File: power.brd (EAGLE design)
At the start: 136 x 136 mm, 35 parts, among them CN1 21700, CN2 21700, CN3 21700, CN4 21700, CN5 15PIN 0.5MM, Q6 IRLML6244, Q7 IRLML6244, U17 MAX17320G20+

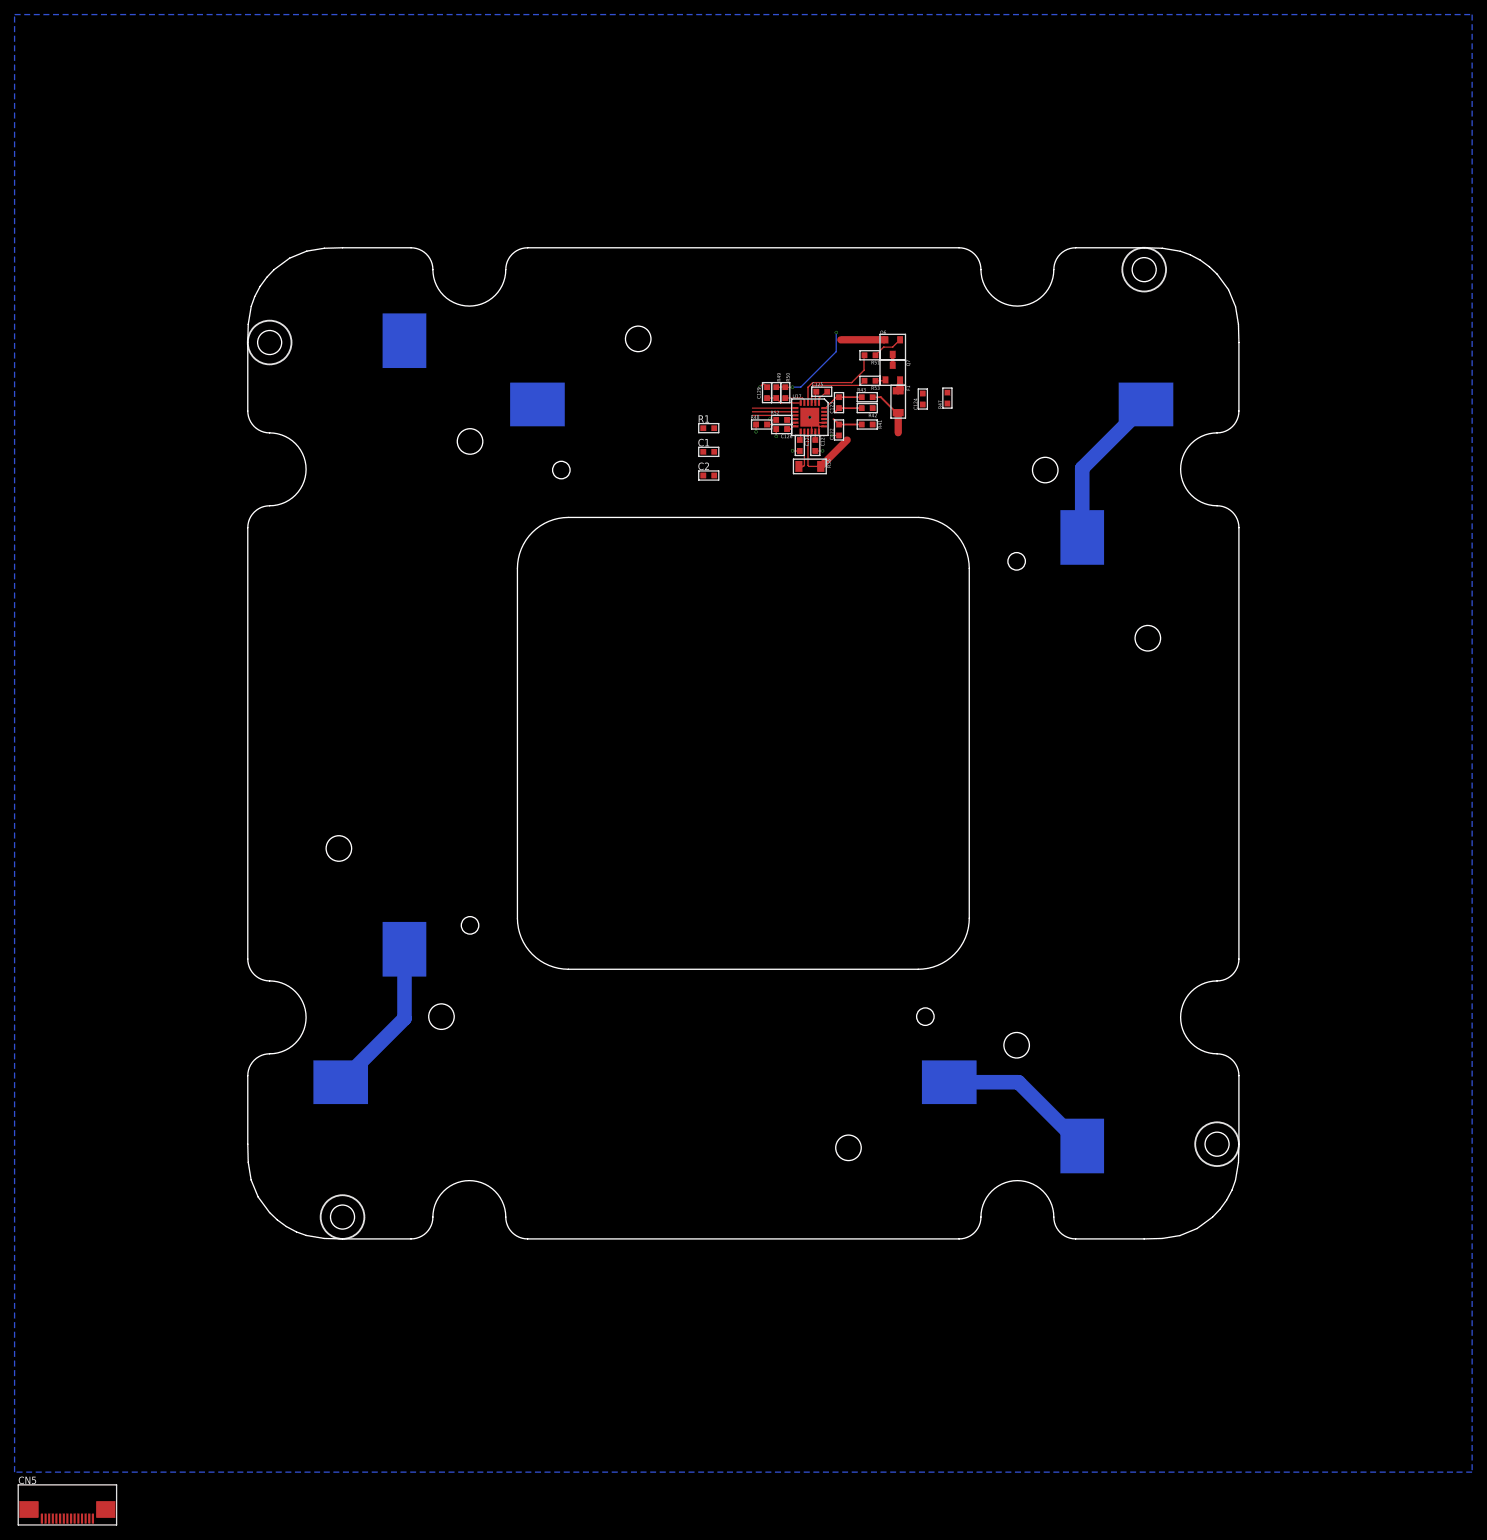
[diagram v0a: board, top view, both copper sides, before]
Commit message: Mech design and layout
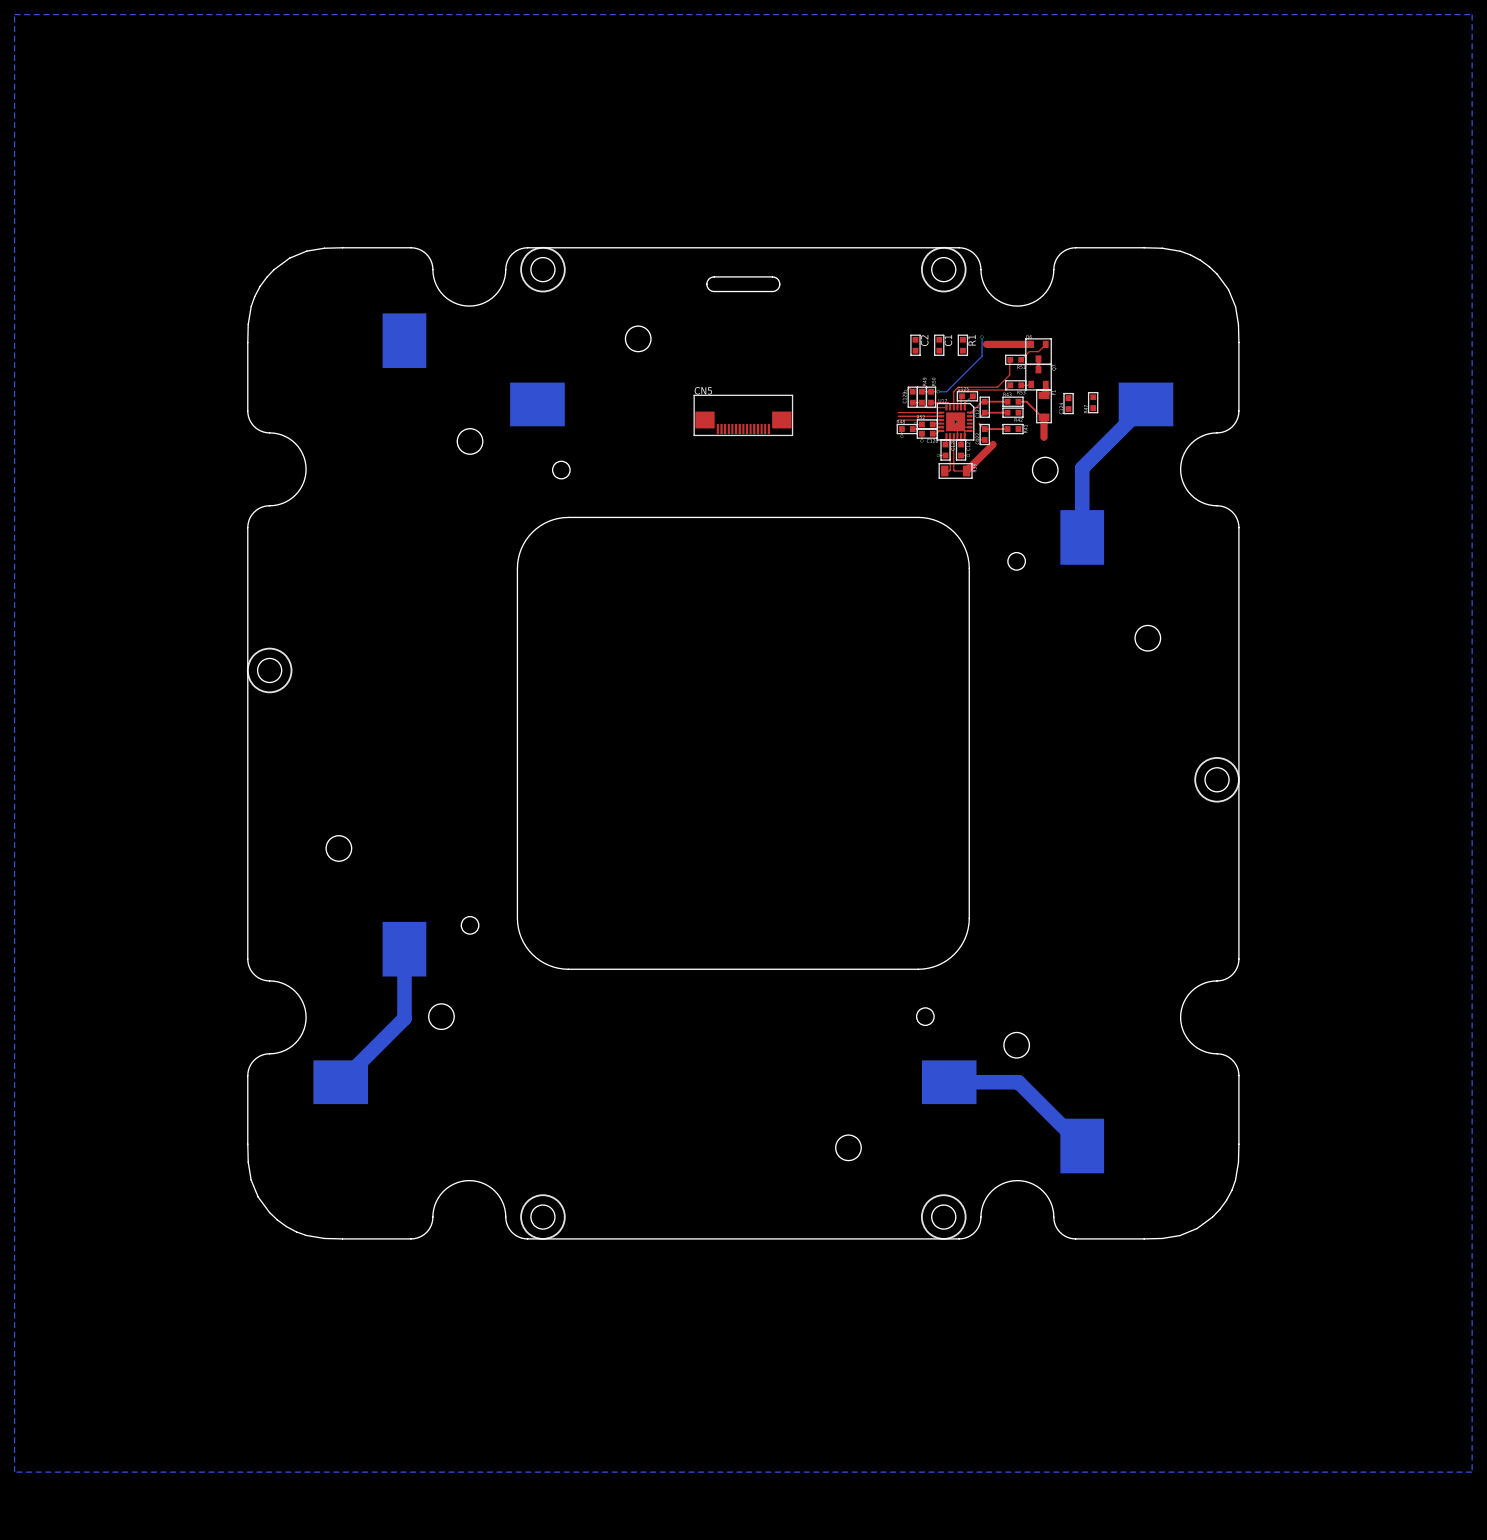
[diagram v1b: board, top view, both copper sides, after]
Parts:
- added MECH5, MECH6: 6mm x 3mm, MISC:MOUNTHOLE_6X3
- moved CN5 175.9 mm to (0.00, 45.0)
- moved MECH2 38.8 mm to (-27.5, 65.0)
- moved MECH4 38.8 mm to (27.5, -65.0)
- moved R1 36.7 mm to (30.1, 54.6), turned to 270 degrees
- moved C1 34.8 mm to (26.9, 54.6), turned to 270 degrees
- moved C2 33.5 mm to (23.6, 54.6), turned to 270 degrees
- moved MECH1 27.5 mm to (-27.5, -65.0)
- moved MECH3 27.5 mm to (27.5, 65.0)
- moved C122 20.0 mm to (33.1, 42.4)
- moved C123 20.0 mm to (33.1, 46.1)
- moved C124 20.0 mm to (44.6, 46.6)
- moved C125 20.0 mm to (30.8, 47.6)
- moved C126 20.0 mm to (25.2, 42.5)
- moved C127 20.0 mm to (29.9, 40.2)
- moved C128 20.0 mm to (27.8, 40.2)
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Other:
- outline, holes or cut-outs redrawn

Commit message: Battery PCB done
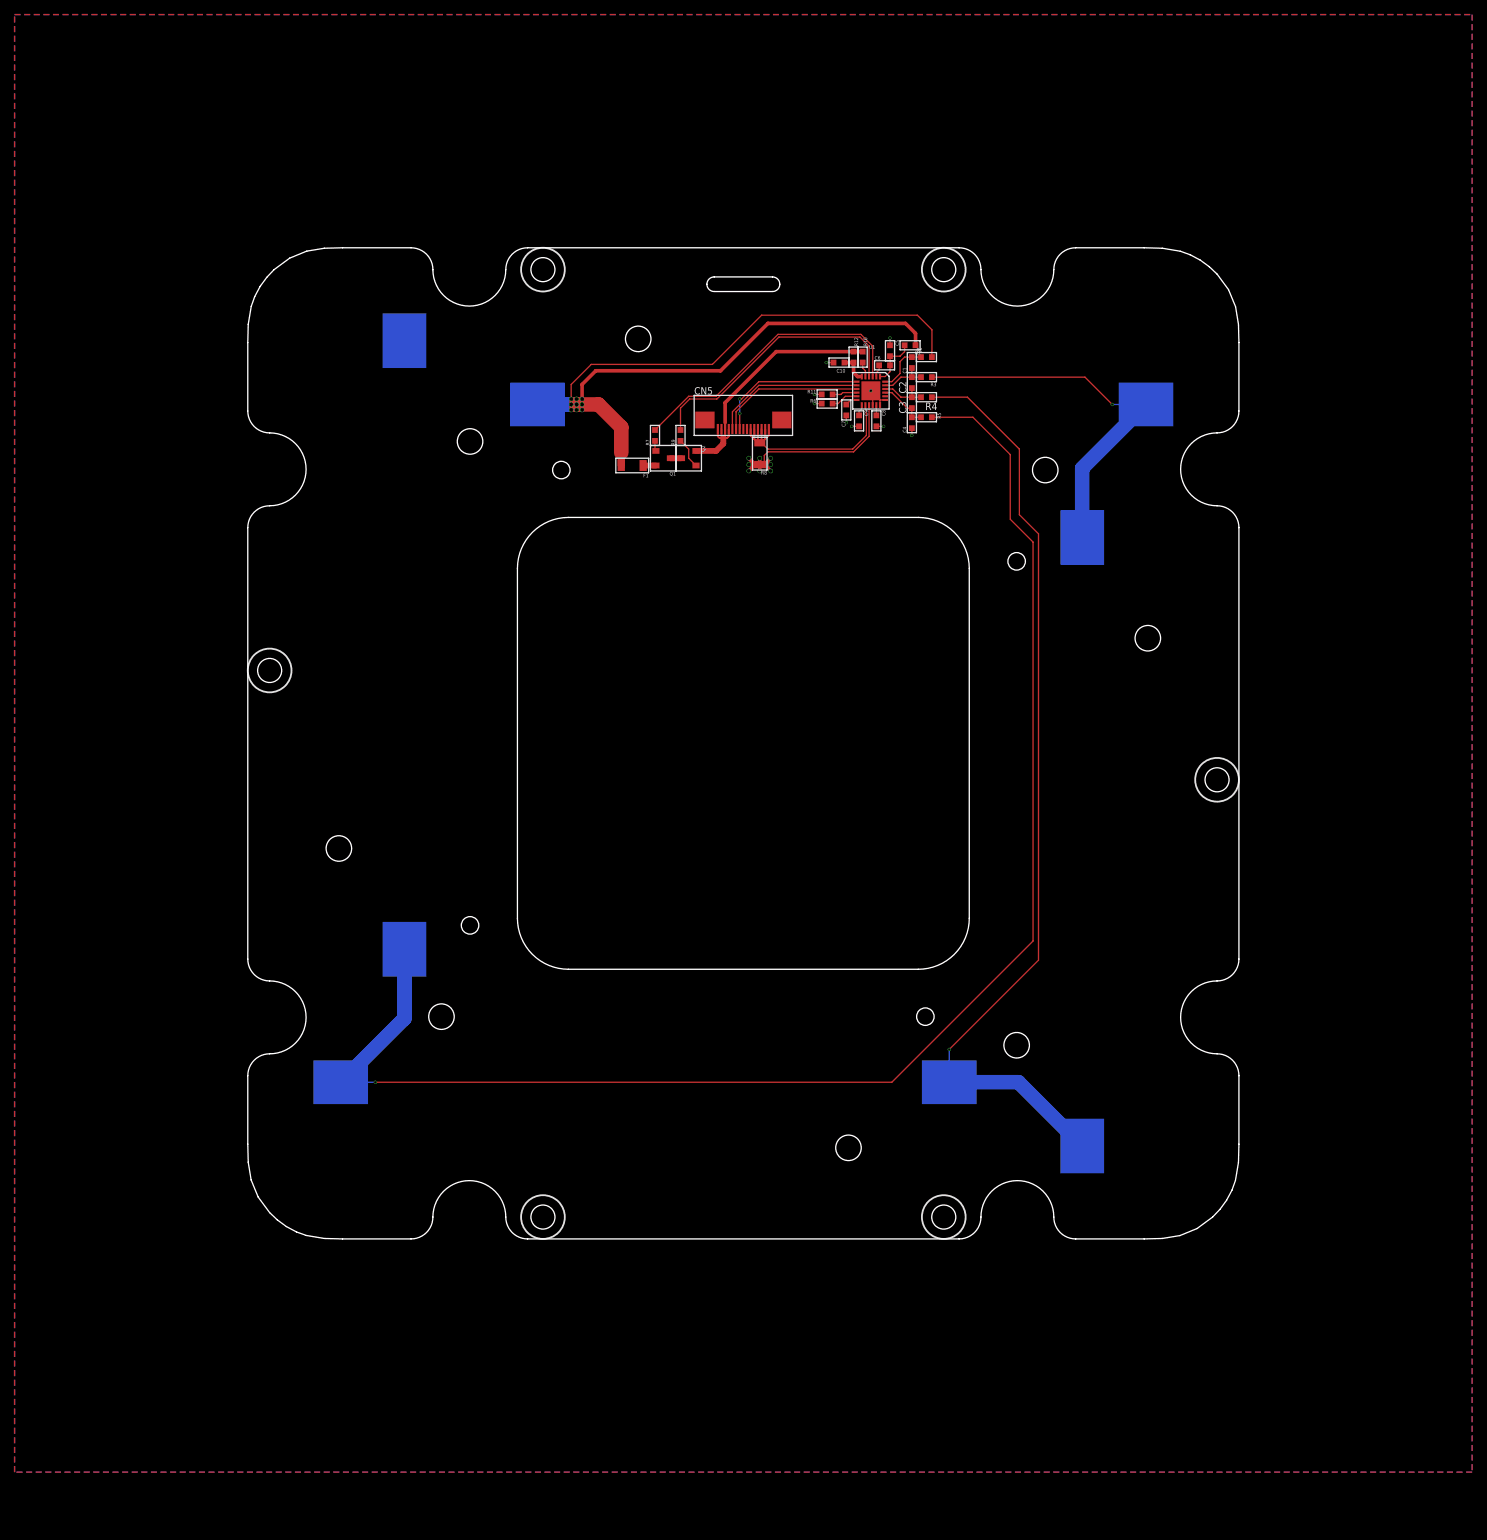
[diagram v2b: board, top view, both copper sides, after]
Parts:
- removed C122, C123, C124: 100nF 16V, CAPACITORS:0603
- removed C125, C126, C127, C128: 470nF 25V, CAPACITORS:0603
- removed C129: 10nF 50V, CAPACITORS:0603
- removed Q6, Q7: IRLML6244, TRANSISTORs:SOT23-3
- removed R38: 0R01, RESISTORS:1206
- removed R41, R42, R43: 47R, r_0603:0603
- removed R47: 10R, r_0603:0603
- removed R48, R49, R50: 1.0k, r_0603:0603
- removed R51, R53: 100R, r_0603:0603
- removed R52: 10k, r_0603:0603
- removed U17: MAX17320G20+, ICs:TQFN24
- added C10: 10nF 50V, CAPACITORS:0603
- added C3, C4, C5: 100nF 16V, CAPACITORS:0603
- added C6, C7, C8, C9: 470nF 25V, CAPACITORS:0603
- added Q1, Q2: IRLML6244, TRANSISTORs:SOT23-3
- added R10, R12, R6: 1.0k, r_0603:0603
- added R11: 10k, r_0603:0603
- added R2, R3, R4, R5: 47R, r_0603:0603
- added R7, R9: 100R, r_0603:0603
- added R8: 0R01, RESISTORS:1206
- added U1: MAX17320G20+, ICs:TQFN24
- R1: value 47R -> 10R
- moved MECH4 141.2 mm to (-27.5, 65.0)
- moved MECH5 119.1 mm to (27.5, -65.0)
- moved MECH3 107.6 mm to (-65.0, 10.0)
- moved F1 57.1 mm to (-15.2, 38.1), turned to 180 degrees
- moved MECH2 55.0 mm to (27.5, 65.0)
- moved R1 7.25 mm to (22.9, 54.6), turned to 180 degrees
- moved C2 5.15 mm to (23.1, 49.5), turned to 90 degrees
- moved C1 4.44 mm to (23.1, 52.2), turned to 90 degrees
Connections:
- net BMS_I2C_SCL: now also U1.8; no longer U17.8
- net BMS_I2C_SDA: now also U1.9; no longer U17.9
- net BMS_NALERT: now also U1.7; no longer U17.7
- net BMS_TH1: now also R11.2, U1.10; no longer R52.2, U17.10
- net GND: now also R8.1, U1.14; no longer C126.2, C129.1, R38.1, U17.14
- net N$1: now also C3.1, C4.2, R5.2, U1.21; no longer C1.1, C122.2, R41.2, U17.21
- net N$2: now also C1.1, R3.2, U1.23; no longer C123.1, R42.2, U17.23
- net N$3: now also C3.2, R4.2, U1.22; no longer C1.2, R1.2, U17.22
- net N$36: now also R1.1, R2.1; no longer R43.1, R47.1
- net N$38: now also C5.2, C6.1, R1.2, U1.1; no longer C124.2, C125.1, R47.2, U17.1
- net N$39: now also C1.2, R2.2, U1.24; no longer C123.2, R43.2, U17.24
- net N$4: now also R3.1; no longer R42.1
- net N$41: now also C6.2, U1.2; no longer C125.2, U17.2
- net N$42: now also Q1.3; no longer Q7.3
- net N$43: now also Q2.1, R9.2; no longer Q6.1, R51.2
- net N$45: now also R6.2, U1.11; no longer R48.2, U17.11
- net N$46: now also C10.2, R12.1, U1.6; no longer C129.2, R49.1, U17.6
- net N$47: now also R10.1, U1.5; no longer R50.1, U17.5
- net N$48: now also C7.1, U1.12; no longer C126.1, U17.12
- net N$49: now also C8.1, U1.17; no longer C127.1, U17.17
- net N$5: now also R4.1; no longer R1.1
- net N$55: now also C9.1, U1.13; no longer C128.1, U17.13
- net N$56: now also R9.1, U1.4; no longer R51.1, U17.4
- net N$57: now also Q1.2, Q2.2; no longer Q6.2, Q7.2
- net N$58: now also Q1.1, R7.2; no longer Q7.1, R53.2
- net N$59: now also R7.1, U1.3; no longer R53.1, U17.3
- net PACK_MID: now also R5.1; no longer R41.1
- net PGND: now also C10.1, C4.1, C5.1, C7.2, C8.2, C9.2, R11.1, R6.1, R8.2, U1.15, U1.16, U1.18, U1.19, U1.20, U1.PAD; no longer C122.1, C124.1, C127.2, C128.2, R38.2, R48.1, R52.1, U17.15, U17.16, U17.18, U17.19, U17.20, U17.PAD
- net PWR_VPACK: now also Q2.3, R10.2, R12.2; no longer Q6.3, R49.2, R50.2
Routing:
- net PACK_MID: track 21.9 -> 205.8 mm, vias 0 -> 1
- net N$36: track 7.13 -> 141.5 mm, vias 0 -> 9
- net N$5: track 21.9 -> 129.9 mm, vias 0 -> 1
- net N$4: track 21.9 -> 52.8 mm, vias 0 -> 1
- net N$59: track 9.78 -> 40.2 mm
- net N$56: track 13.2 -> 37.6 mm
- net GND: track 7.89 -> 31.5 mm, vias 2 -> 0
- net PGND: track 22.6 -> 44.3 mm, vias 6 -> 17
- net PWR_VPACK: track 19.0 -> 36.7 mm, vias 2 -> 0
- net BMS_NALERT: track 5.92 -> 21.2 mm, vias 0 -> 2
- net BMS_I2C_SCL: track 5.92 -> 20.9 mm
- net BMS_I2C_SDA: track 5.92 -> 20.2 mm
- net N$3: track 0.00 -> 6.74 mm
- net N$38: track 2.10 -> 6.91 mm
- net N$1: track 4.19 -> 7.05 mm
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- added copper zone on layer 1, net PGND
